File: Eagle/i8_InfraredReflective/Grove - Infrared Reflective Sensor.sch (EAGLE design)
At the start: 11 parts, among them U1 002-LMV358

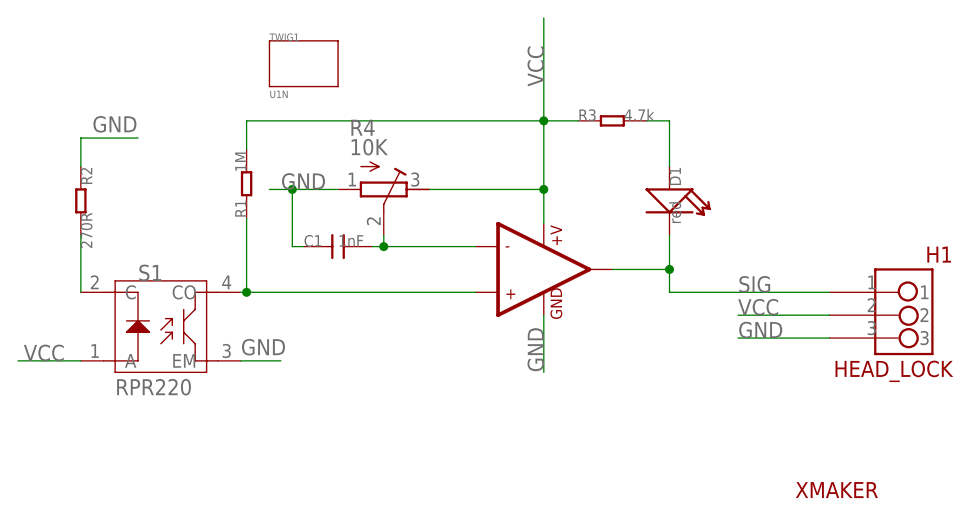
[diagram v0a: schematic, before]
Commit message: 第一次更新
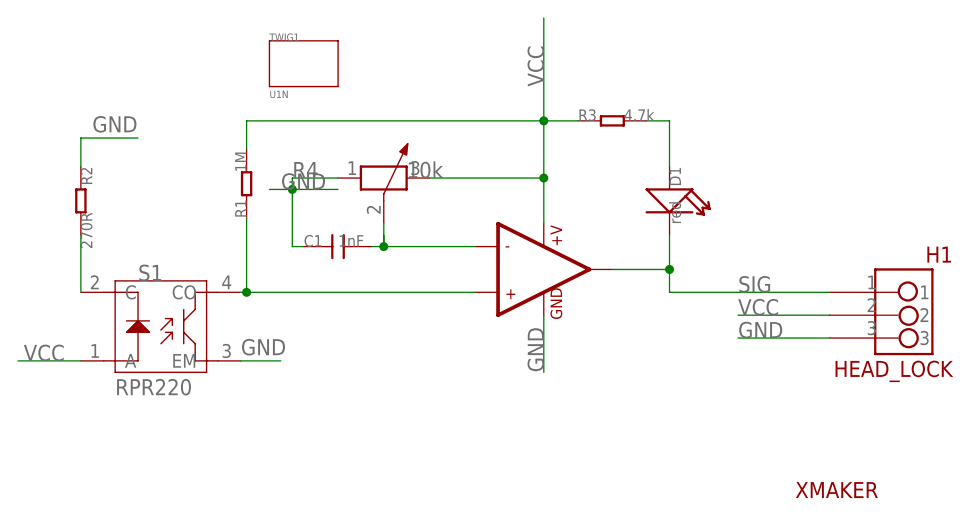
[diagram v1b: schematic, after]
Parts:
- R4: value 10K -> 10k; device rcl:R-TRIMM3214W -> Discrete:R-POTENTIOMETEREVN-D8A-A03-B**
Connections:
- net GND: now also R4.1; no longer R4.E
- net N$1: now also R4.3; no longer R4.S
- net VCC: now also R4.2; no longer R4.A
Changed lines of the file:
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@@
 <?xml version="1.0" encoding="utf-8"?>
 <!DOCTYPE eagle SYSTEM "eagle.dtd">
-<eagle version="7.2.0">
+<eagle version="6.6.0">
 <drawing>
 <settings>
@@
 <setting verticaltext="up"/>
 </settings>
-<grid distance="0.1" unitdist="inch" unit="inch" style="lines" multiple="1" display="no" altdistance="0.01" altunitdist="inch" altunit="inch"/>
+<grid distance="10" unitdist="mil" unit="mil" style="lines" multiple="1" display="no" altdistance="0.01" altunitdist="inch" altunit="inch"/>
 <layers>
 <layer number="1" name="Top" color="4" fill="1" visible="no" active="no"/>
@@
 <layer number="90" name="Modules" color="5" fill="1" visible="no" active="no"/>
 <layer number="91" name="Nets" color="2" fill="1" visible="yes" active="yes"/>
-<layer number="92" name="Busses" color="1" fill="1" visible="no" active="yes"/>
+<layer number="92" name="Busses" color="1" fill="1" visible="yes" active="yes"/>
 <layer number="93" name="Pins" color="2" fill="1" visible="no" active="yes"/>
 <layer number="94" name="Symbols" color="4" fill="1" visible="yes" active="yes"/>
@@
 </classes>
 <parts>
-<part name="R4" library="rcl" deviceset="R-TRIMM" device="3214W" value="10K"/>
 <part name="U1" library="ICs" deviceset="002-LMV358" device=""/>
 <part name="D1" library="Discrete" deviceset="007-LED*" device="35*40" value="red"/>
@@
 <part name="H1" library="HEAD_LOCK" deviceset="HEAD_LOCK" device=""/>
 <part name="U$3" library="Xmaker_yuhui" deviceset="XMAKERLOGO2" device=""/>
+<part name="R4" library="Discrete" deviceset="R-POTENTIOMETER*" device="EVN-D8A-A03-B**" value="10k"/>
 </parts>
 <sheets>
@@
 </plain>
 <instances>
-<instance part="R4" gate="G$1" x="109.22" y="80.01" rot="R270"/>
 <instance part="U1" gate="G$1" x="127" y="71.12"/>
 <instance part="D1" gate="LED" x="140.97" y="78.74" rot="R270"/>
@@
 <instance part="H1" gate="G$1" x="171.45" y="58.42" rot="MR0"/>
 <instance part="U$3" gate="G$1" x="160.02" y="48.26"/>
+<instance part="R4" gate="RP" x="109.22" y="81.28"/>
 </instances>
 <busses>
@@
 <net name="VCC" class="0">
 <segment>
-<wire x1="127" y1="76.2" x2="127" y2="80.01" width="0.1524" layer="91"/>
-<wire x1="127" y1="80.01" x2="127" y2="87.63" width="0.1524" layer="91"/>
+<wire x1="127" y1="76.2" x2="127" y2="81.28" width="0.1524" layer="91"/>
+<wire x1="127" y1="81.28" x2="127" y2="87.63" width="0.1524" layer="91"/>
 <wire x1="127" y1="87.63" x2="127" y2="99.06" width="0.1524" layer="91"/>
-<wire x1="114.3" y1="80.01" x2="127" y2="80.01" width="0.1524" layer="91"/>
 <wire x1="93.98" y1="87.63" x2="127" y2="87.63" width="0.1524" layer="91"/>
 <wire x1="130.81" y1="87.63" x2="127" y2="87.63" width="0.1524" layer="91"/>
-<junction x="127" y="80.01"/>
 <junction x="127" y="87.63"/>
 <label x="127" y="91.44" size="1.778" layer="95" rot="R90"/>
 <pinref part="U1" gate="G$1" pin="+V"/>
-<pinref part="R4" gate="G$1" pin="A"/>
 <pinref part="R3" gate="R" pin="1"/>
 <pinref part="R1" gate="R" pin="2"/>
 <wire x1="93.98" y1="84.455" x2="93.98" y2="87.63" width="0.1524" layer="91"/>
+<pinref part="R4" gate="RP" pin="2"/>
+<wire x1="114.3" y1="81.28" x2="127" y2="81.28" width="0.1524" layer="91"/>
+<junction x="127" y="81.28"/>
 </segment>
 <segment>
@@
 <wire x1="109.22" y1="74.93" x2="109.22" y2="73.66" width="0.1524" layer="91"/>
 <wire x1="109.22" y1="73.66" x2="119.38" y2="73.66" width="0.1524" layer="91"/>
-<pinref part="R4" gate="G$1" pin="S"/>
 <pinref part="U1" gate="G$1" pin="-IN1"/>
 <pinref part="C1" gate="C" pin="2"/>
 <wire x1="109.22" y1="73.66" x2="107.95" y2="73.66" width="0.1524" layer="91"/>
 <junction x="109.22" y="73.66"/>
+<pinref part="R4" gate="RP" pin="3"/>
+<wire x1="109.22" y1="76.2" x2="109.22" y2="73.66" width="0.1524" layer="91"/>
 </segment>
 </net>
@@
 </segment>
 <segment>
-<pinref part="R4" gate="G$1" pin="E"/>
 <wire x1="104.14" y1="80.01" x2="99.06" y2="80.01" width="0.1524" layer="91"/>
 <label x="97.79" y="80.01" size="1.778" layer="95"/>
@@
 <wire x1="99.06" y1="73.66" x2="99.06" y2="80.01" width="0.1524" layer="91"/>
 <junction x="99.06" y="80.01"/>
-</segment>
-<segment>
+<pinref part="R4" gate="RP" pin="1"/>
+<wire x1="99.06" y1="81.28" x2="104.14" y2="81.28" width="0.1524" layer="91"/>
+<wire x1="99.06" y1="81.28" x2="99.06" y2="80.01" width="0.1524" layer="91"/>
+</segment>
+<segment>
